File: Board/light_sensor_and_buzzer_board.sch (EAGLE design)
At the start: 5 parts, among them U1 TEM-HUM-AM2302(4P-25.0X15.0MM)

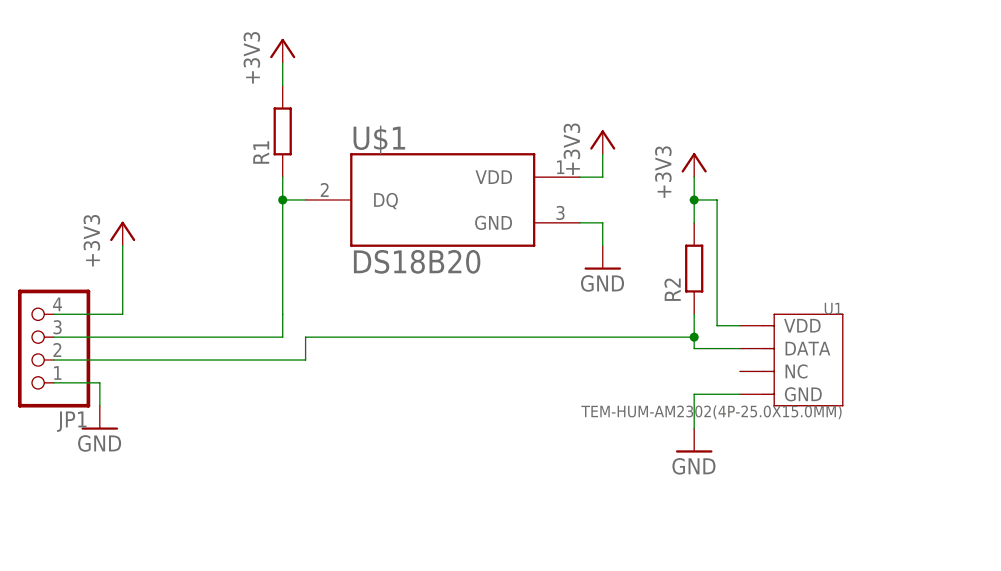
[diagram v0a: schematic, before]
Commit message: Update
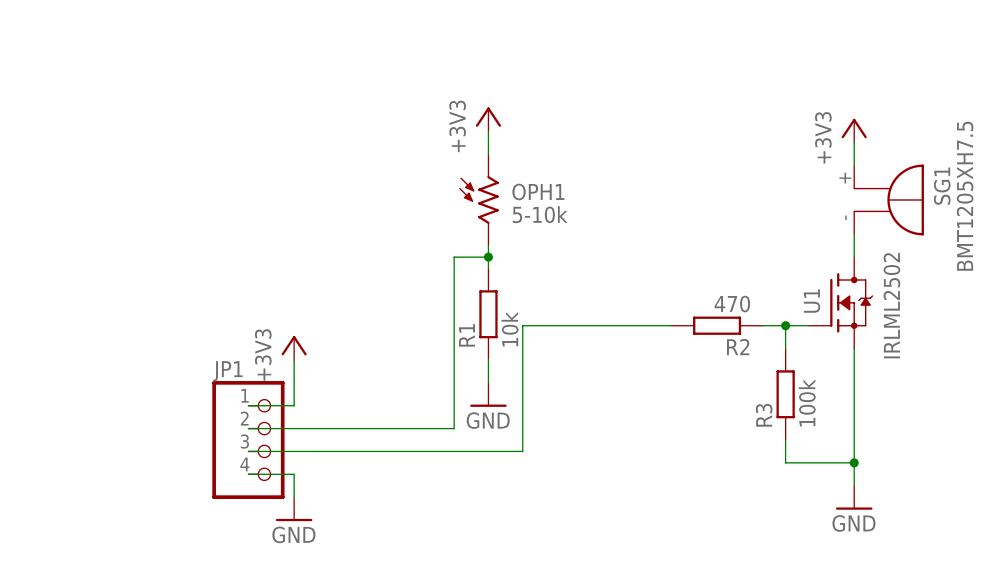
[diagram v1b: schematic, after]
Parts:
- removed U$1: DS18B20, DS18B20_PAR:DS18B20
- added OPH1: 5-10k, photo-elements:VT90N1
- added R3: 100k, rcl:R-EU_R1206
- added SG1: BMT1205XH7.5, buzzer:BMT1205XH7.5
- R1: value (none) -> 10k
- R2: value (none) -> 470
- U1: value TEM-HUM-AM2302(4P-25.0X15.0MM) -> IRLML2502; device TEM-HUM-AM2302_4P-25.0X15.0MM_:TEM-HUM-AM2302(4P-25.0X15.0MM) -> IRLML2502TRPBF:IRLML2502TRPBF
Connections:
- new net N$3: R2.1, R3.2, U1.G
- new net N$4: JP1.3, R2.2
- net +3V3: now also JP1.1, OPH1.1, SG1.+; no longer JP1.4, R1.2, R2.2, U$1.VDD, U1.VDD
- net GND: now also JP1.4, R1.1, R3.1, U1.S; no longer JP1.1, U$1.GND, U1.GND
- net N$1: now also OPH1.2, R1.2; no longer R2.1, U1.DATA
- net N$2: now also SG1.-, U1.D; no longer JP1.3, R1.1, U$1.DQ
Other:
- moved on the sheet: JP1, R1, R2
